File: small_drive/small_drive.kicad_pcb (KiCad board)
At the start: 2 copper layers, 100 x 100 mm, 155 parts, among them J1 DB9, J2 DB15, M1 SiR826DP, M2 SiR826DP, M3 SiR826DP, M4 SiR826DP, M5 SiR826DP, M6 SiR826DP, P1 CONN_01X04, P2 CONN_01X04, P3 CONN_01X04, P5 CONN_01X02, P6 CONN_01X02, P7 CONN_01X02, U1 XMC4400-F64x512, U10 LM5106, U11 ACS711KLCTR-12AB-T, U12 ACS711ELCTR-25AB-T, U13 ACS711KLCTR-12AB-T, U14 AD8226, U15 MAX3096, U16 AMC1203, U17 7805, U18 LT1764EQ, U19 KSZ8081, U2 ips511g, U20 ETH100_MAG, U3 ips511g, U4 LTC2850, U5 AD8226, U6 LT1764EQ, U7 MC33074DTBR2, U8 LM5106, U9 LM5106, X1 NKE1212DC, X2 NKE1212DC, X3 HCPL0201, X4 HCPL0201, X5 HCPL0201, X6 HCPL0201, Y1 12MHz, Y2 25MHz

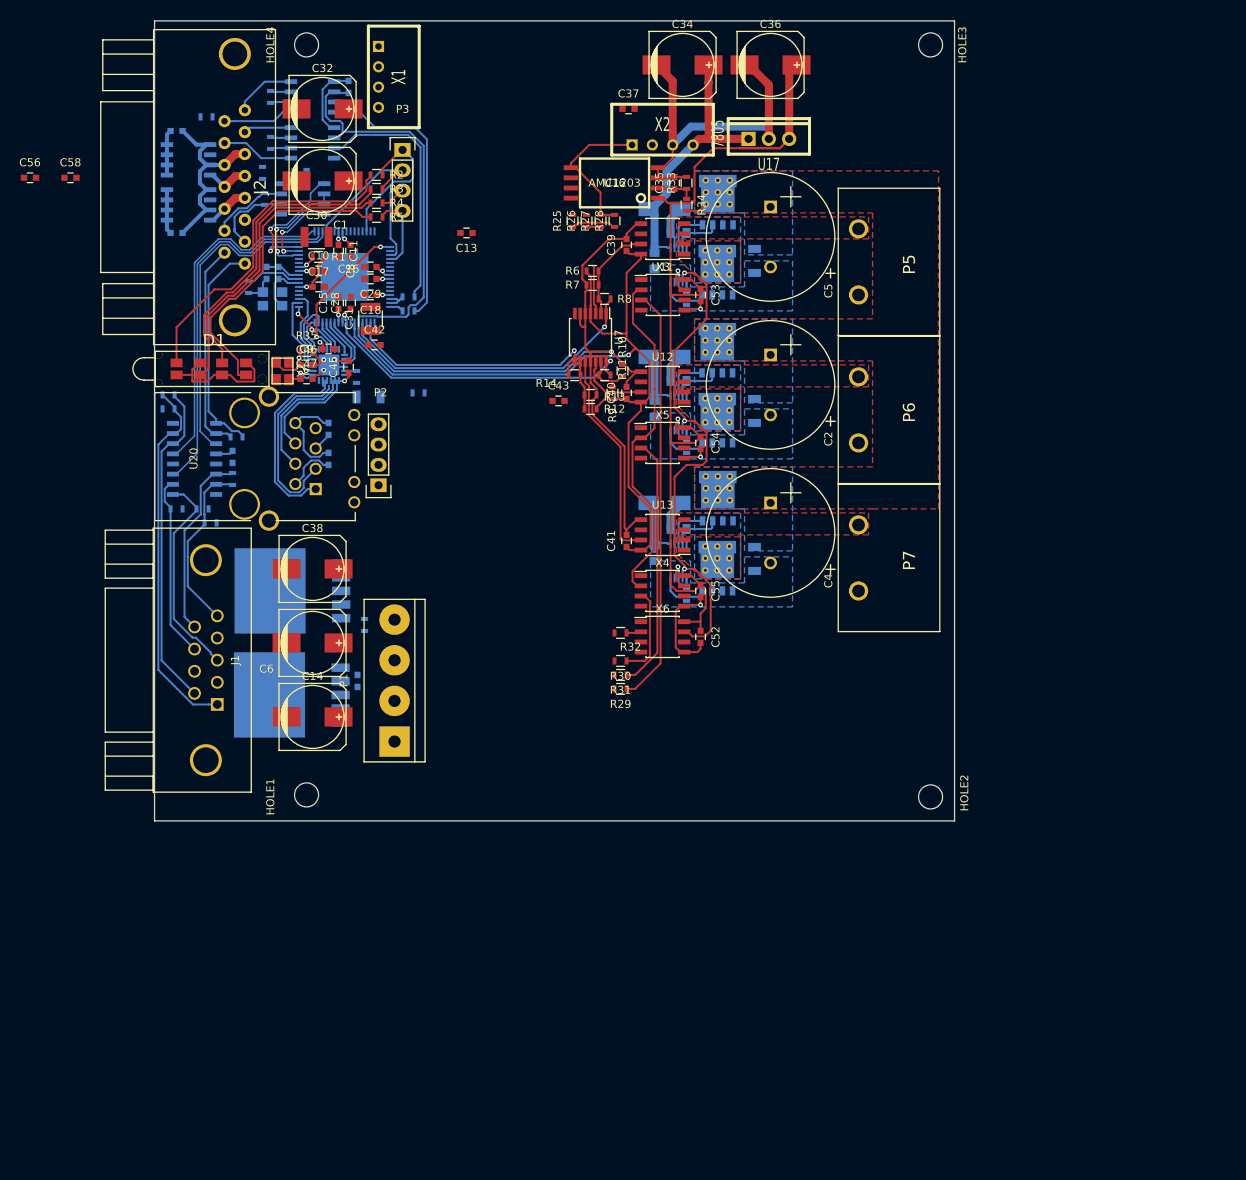
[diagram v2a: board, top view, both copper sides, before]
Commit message: Pauze backup
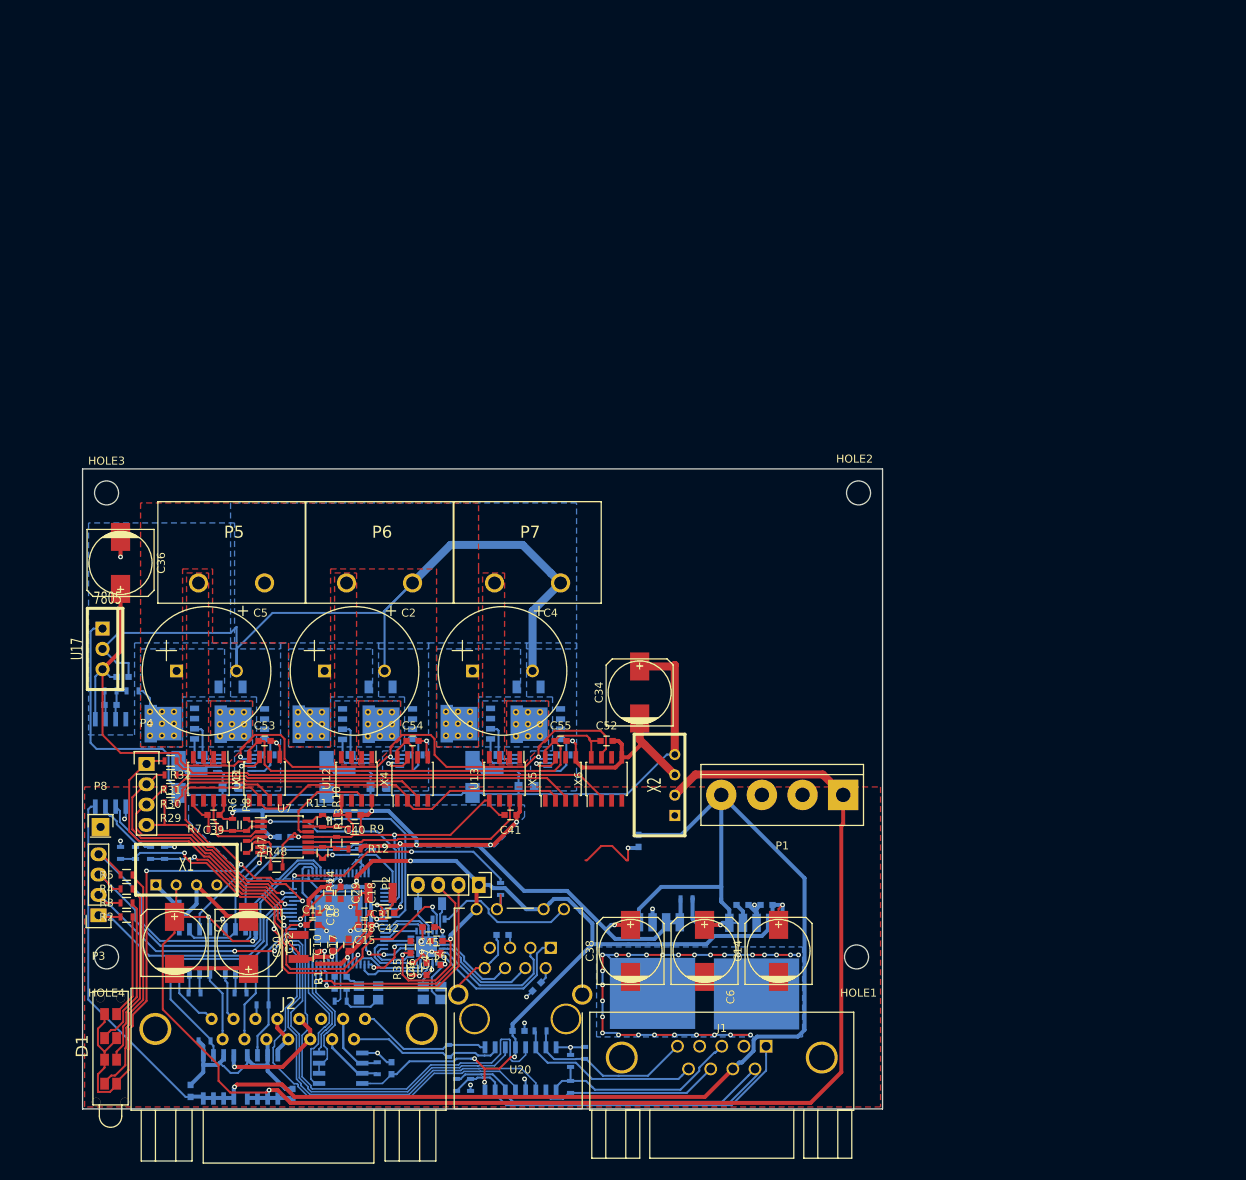
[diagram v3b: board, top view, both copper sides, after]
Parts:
- added P4: CONN_01X04, Pin_Headers:Pin_Header_Straight_1x04, F.Cu at (47.0, 140.9)
- added P8: CONN_01X01, Pin_Headers:Pin_Header_Straight_1x01, F.Cu at (41.2, 148.8)
- added R47: 10k, Resistors_SMD:R_0603, F.Cu at (59.5, 151.2)
- added R48: 10k, Resistors_SMD:R_0603, F.Cu at (63.2, 153.8)
- C13, C35, C37, C43, C58, R25, R26, R27, R28, R33, R34, U16, Y2: moved to B.Cu
- P1: footprint Connect:bornier4 -> 00_Passives:PC_drive_5.25_conn
- moved C3 121.4 mm to (65.2, 182.2), turned to 90 degrees
- moved C58 118.3 mm to (77.6, 178.9), turned to 90 degrees
- moved HOLE3 117.2 mm to (42.0, 107.0), turned to 90 degrees
- moved HOLE4 116.7 mm to (42.0, 165.0), turned to 90 degrees
- moved U3 115.0 mm to (61.5, 180.0), turned to 270 degrees
- moved R22 112.4 mm to (53.0, 169.5), turned to 180 degrees
- moved R19 111.2 mm to (61.5, 171.0), turned to 180 degrees
- moved R21 109.6 mm to (75.8, 178.9), turned to 90 degrees
- moved U2 109.1 mm to (56.0, 180.0), turned to 270 degrees
- moved U4 108.8 mm to (71.3, 178.9), turned to 0 degrees
- moved R20 108.7 mm to (54.2, 175.5), turned to 180 degrees
- moved C59 108.7 mm to (124.5, 158.5), turned to 180 degrees
- moved C56 108.1 mm to (83.2, 163.0), turned to 180 degrees
- moved U5 107.8 mm to (53.0, 164.2), turned to 90 degrees
- moved C7 107.3 mm to (52.5, 181.8), turned to 90 degrees
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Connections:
- R2 pad 1: Net-(D1-Pad8) -> Net-(D1-Pad4)
- R3 pad 1: Net-(D1-Pad2) -> Net-(D1-Pad6)
- R4 pad 1: Net-(D1-Pad6) -> Net-(D1-Pad2)
- R5 pad 1: Net-(D1-Pad4) -> Net-(D1-Pad8)
- U1 pad 53: /ENC_5V -> /ENC_12V
- U1 pad 59: /ENC_12V -> /ENC_5V
- U1 pad 60: /HB1 -> /HB2
- U1 pad 63: /HB2 -> /HB1
- U14 pad 6: GND -> Net-(U14-Pad6)
- U16 pad 2: Net-(C35-Pad1) -> GNDPWR
- U16 pad 3: GNDPWR -> Net-(C35-Pad1)
- U5 pad 6: GND -> Net-(U14-Pad6)
- U7 pad 5: GND -> Net-(R47-Pad2)
- U7 pad 6: GND -> Net-(U14-Pad6)
- U7 pad 7: Net-(U7-Pad7) -> Net-(U14-Pad6)
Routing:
- net +3.3V: track 77.8 -> 317.3 mm, vias 6 -> 14
- net +5V: track 5.59 -> 211.8 mm, vias 0 -> 2
- net +12V: track 5.71 -> 187.8 mm, vias 0 -> 3
- net GNDPWR: track 65.5 -> 143.0 mm, vias 3 -> 4
- net +12P: track 50.6 -> 122.3 mm
- net /ENC_RXD2: track 0.00 -> 65.8 mm
- net Net-(R32-Pad1): track 1.86 -> 55.6 mm
- net GND: track 222.9 -> 265.0 mm, vias 4 -> 50
- net Net-(R29-Pad1): track 52.3 -> 14.4 mm
- net /HBEN: track 0.00 -> 37.5 mm, vias 0 -> 1
- net /MDAT: track 5.68 -> 42.0 mm, vias 0 -> 2
- net /ETH0_~RST: track 0.00 -> 35.5 mm, vias 0 -> 2
- net /LED3: track 10.0 -> 45.5 mm
- net /ENC_5V: track 0.00 -> 33.7 mm
- net /A: track 41.2 -> 74.6 mm
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- added copper zone on B.Cu, net +3.3VADC
- added copper zone on B.Cu, net GND
- added copper zone on F.Cu, net GND
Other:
- board size 100 x 100 mm -> 100 x 80 mm
